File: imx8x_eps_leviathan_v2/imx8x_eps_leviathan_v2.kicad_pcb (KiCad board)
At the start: 6 copper layers, 100 x 100 mm, 433 parts, among them CN1 DF11-16DP-2DSA(08), CN2 DF11-16DP-2DSA(08), CN3 DF11-16DP-2DSA, J1 Conn_01x01_Socket, J2 Conn_01x01_Socket, J3 Conn_01x01_Socket, J4 Conn_01x01_Socket, J6 BTH-070-02-L-D-A, J7 BTH-070-02-L-D-A, Q1 IRLML6401, Q2 BSS138, SW1 SW_DIP_x01, SW2 KMR221GLFS, T1 WE-RJ45_7499111121A, T2 WE-RJ45_7499111121A, U1 XT60PW-F_C428722, U10 TCA4307DGKR, U11 LT8612EUDE#PBF, U12 INA260AIPWR, U13 TPS1HB08BQPWPRQ1, U14 LT8612EUDE#PBF, U15 INA260AIPWR, U16 TLV1704, U17 TLV1704, U18 BD2204GUL-E2, U19 CAT93C66VI-GT3, U2 MCP9808T-E/MS, U20 FT2232HL, U21 LP38693MP-ADJ/NOPB, U22 TXS0101DCKR, U23 TXS0101DCKR, U24 MCP1824T-ADJE/OT, U25 DP83867CRRGZR, U26 TLV71310PDQNR, U27 74LVC2G07GW, U28 TCA4307DGKR, U29 TXS0108EPWR, U3 MCP9808T-E/MS, U30 TXS0108EPWR, U31 TPS22917DBVR, U32 TLV62569PDDCR, U4 MCP9808T-E/MS, U5 TPS1HB08BQPWPRQ1, U6 LT8612EUDE#PBF, U7 INA260AIPWR, U8 LTC6902, U9 TPS1HB08BQPWPRQ1, Y1 Crystal_GND24, Y2 25MHz

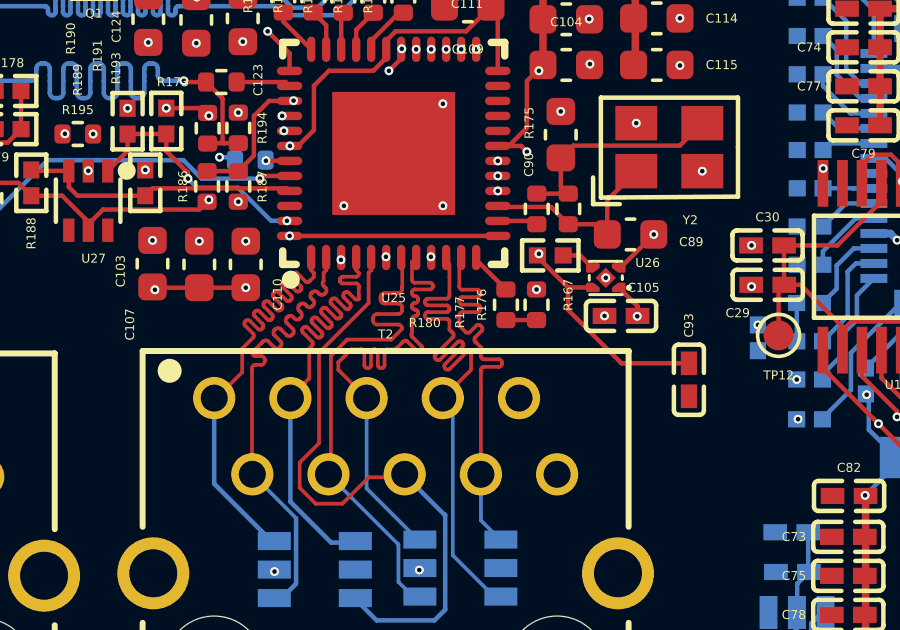
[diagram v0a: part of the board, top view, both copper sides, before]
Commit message: Fixed Duplicates. Updated Gerber and BOM
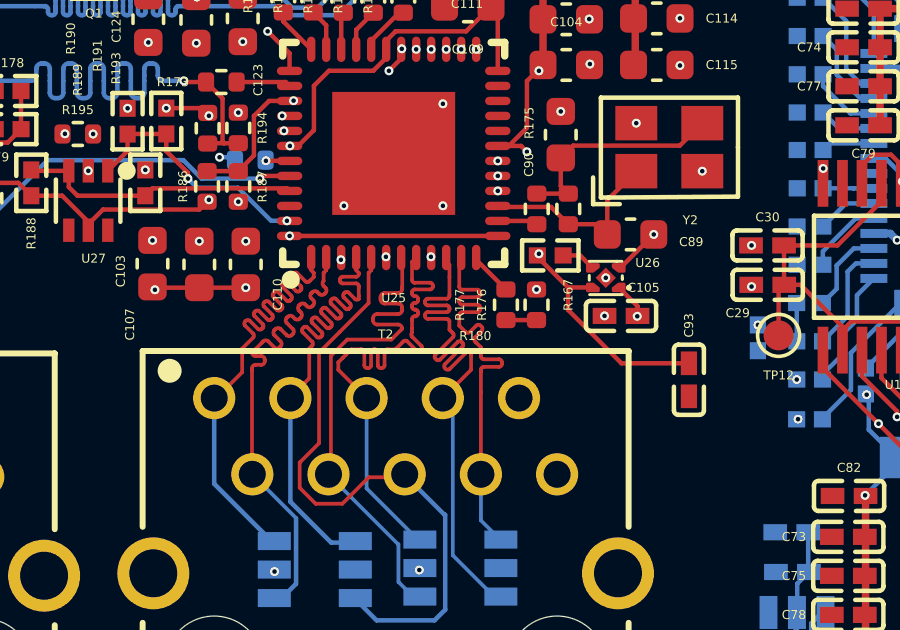
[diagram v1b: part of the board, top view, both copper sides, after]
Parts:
- C100, C104, C106, C111, C112, C117, C121, C130, C85, C92, C94, C98, C99: value 1uF -> 1u
- C101, C102, C103, C105, C108, C109, C113, C119, C122, C61, C63, C68, C69, C74, C75, C76, C77, C78, C79, C80, C82, C84, C86, C87, C88, C91, C93, C95, C96, C97: value 100nF -> 100n
- C107, C114, C116, C123: value 10nF -> 10n
- C110, C115, C120, C124, C133, C64, C65: value 10uF -> 10u
- C118: value 2.2nF -> 2.2n
- C131: value 47uF -> 47u
- C132, C59, C60, C66, C67, C72, C73, C81: value 4.7uF -> 4.7u
- C41, C42, C43: value 100uF -> 100u
- C57, C58: value 22uF -> 22u
- C62: value 220nF -> 220n
- C70, C71: value 12pF -> 12p
- C83: value 2.2uF -> 2.2u
- C89, C90: value 18pF -> 18p
- L6: value 2.2uH -> 2.2u
- R102, R103, R104, R105, R106, R129, R159, R176: value 1K -> 1k
- R107, R108, R109, R110, R111, R112: value 49.9K -> 49.9k
- R120, R121, R123, R124, R127, R132, R133, R134, R135, R136, R137, R138, R139, R140, R141, R142, R143, R144, R147, R148, R149, R150, R151, R152, R153, R154, R155, R156, R157, R158, R160, R161, R162, R163, R166, R177, R180, R181, R188, R192, R195: value 10K -> 10k
- R125, R165, R197: value 2K -> 2k
- R126: value 12K -> 12k
- R164: value 16.5K -> 16.5k
- R168: value 15K -> 15k
- R179: value 13K -> 13k
- R182, R183, R184, R187, R189, R191, R194: value 2.49K -> 2.49k
- R186, R190, R193: value 5.76K -> 5.76k
